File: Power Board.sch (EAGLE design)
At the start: 4 parts

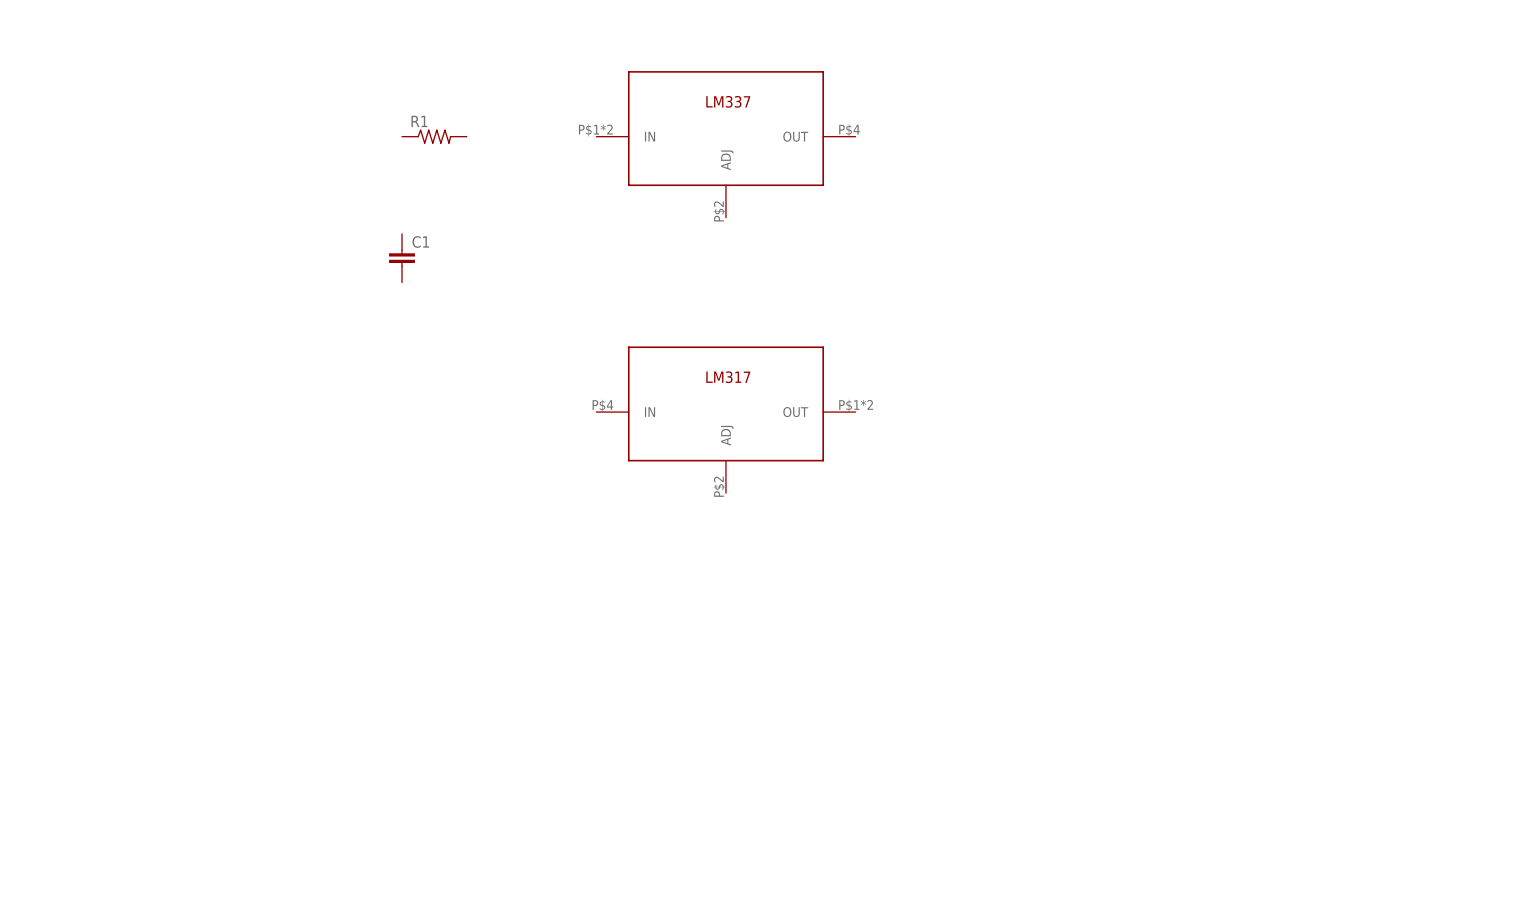
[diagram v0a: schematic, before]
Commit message: Initial layout
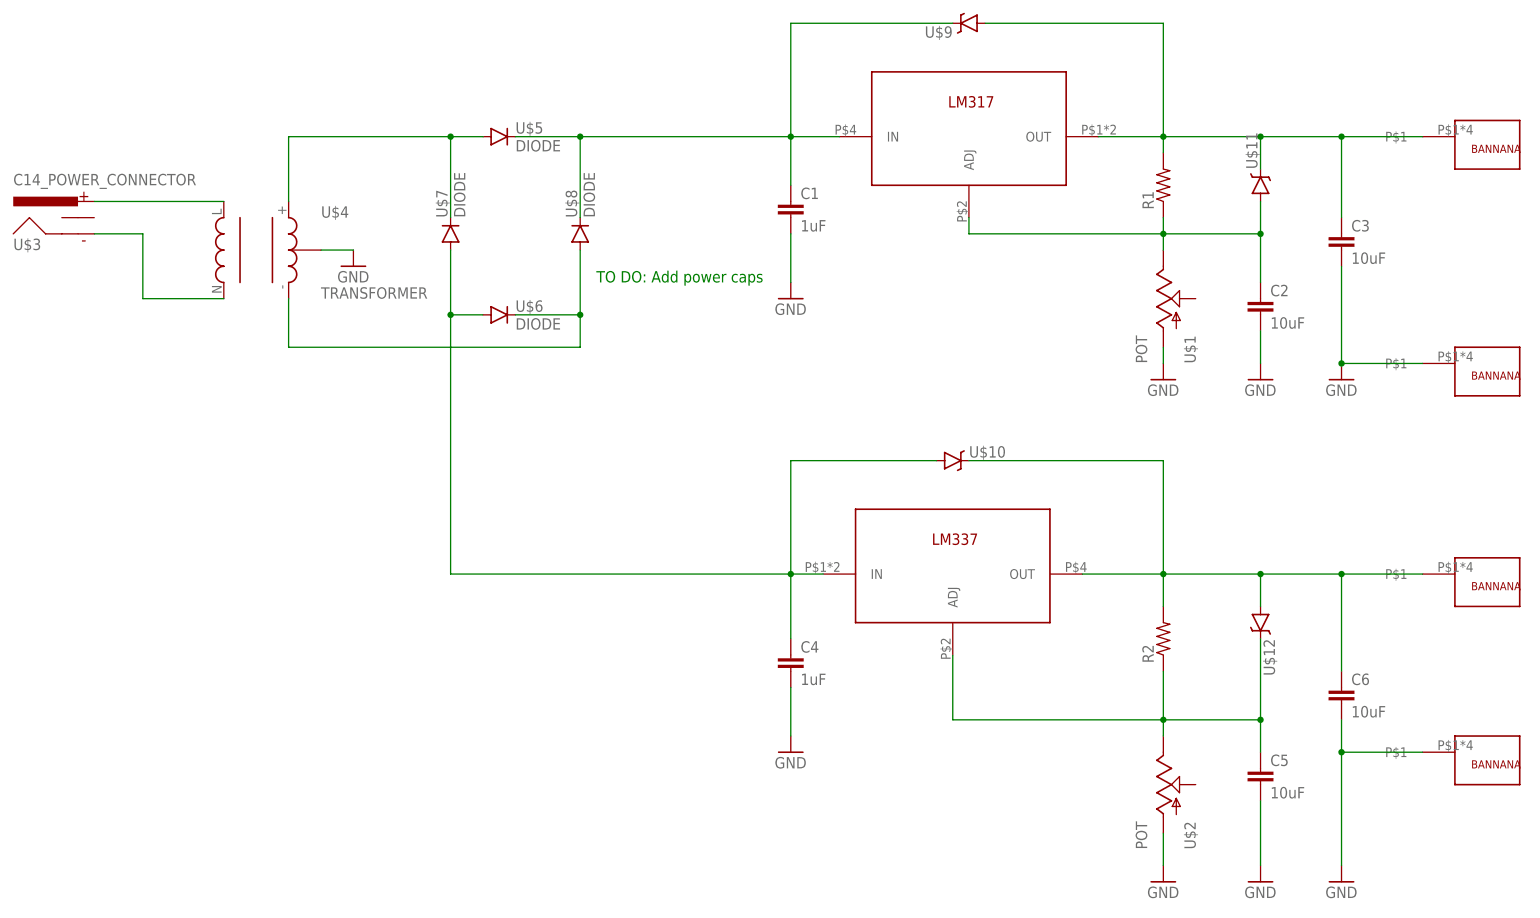
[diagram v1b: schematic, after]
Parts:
- added C2, C3, C5, C6: 10uF, SparkFun-Capacitors:CAP1206
- added C4: 1uF, SparkFun-Capacitors:CAP1206
- added NEG-GND, NEG-OUT, POS-GND, POS-OUT: BANNANA, PowerSupply:BANNANA
- added R2: (no value), SparkFun-Resistors:RESISTOR1206
- added U$1, U$2: POT, PowerSupply:POT
- added U$10, U$11, U$12, U$9: DIODE-SCHOTTKY, PowerSupply:DIODE-SCHOTTKY
- added U$3: C14_POWER_CONNECTOR, PowerSupply:C14_POWER_CONNECTOR
- added U$4: TRANSFORMER, PowerSupply:TRANSFORMER
- added U$5, U$6, U$7, U$8: DIODE, PowerSupply:DIODE
- C1: value (none) -> 1uF
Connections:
- new net GND: C1.2, C2.2, C3.2, C4.2, C5.2, C6.2, U$1.A, U$2.A
- new net N$1: U$3.LINE, U$4.1
- new net N$11: C6.1, LM337.OUT, R2.2, U$10.C, U$12.A
- new net N$12: C5.1, LM337.ADJ, R2.1, U$12.C, U$2.E
- new net N$2: U$3.NEUTRAL, U$4.2
- new net N$3: U$4.5, U$5.A, U$7.C
- new net N$4: C1.1, LM317.IN, U$5.C, U$8.C, U$9.C
- new net N$5: U$4.3, U$6.C, U$8.A
- new net N$6: C3.1, LM317.OUT, R1.2, U$11.C, U$9.A
- new net N$7: C4.1, LM337.IN, U$10.A, U$6.A, U$7.A
- new net N$8: C2.1, LM317.ADJ, R1.1, U$1.E, U$11.A
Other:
- note added: "TO DO: Add power caps"
- moved on the sheet: C1, LM317, LM337, R1
